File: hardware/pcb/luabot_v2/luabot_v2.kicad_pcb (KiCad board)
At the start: 2 copper layers, 60.3 x 29.8 mm, 21 parts, among them CON1 BAT_IN, P2 GND_GPIO, P3 VCC_GPIO, SW1 RESET, U1 ESP-07V2, U2 LM1117

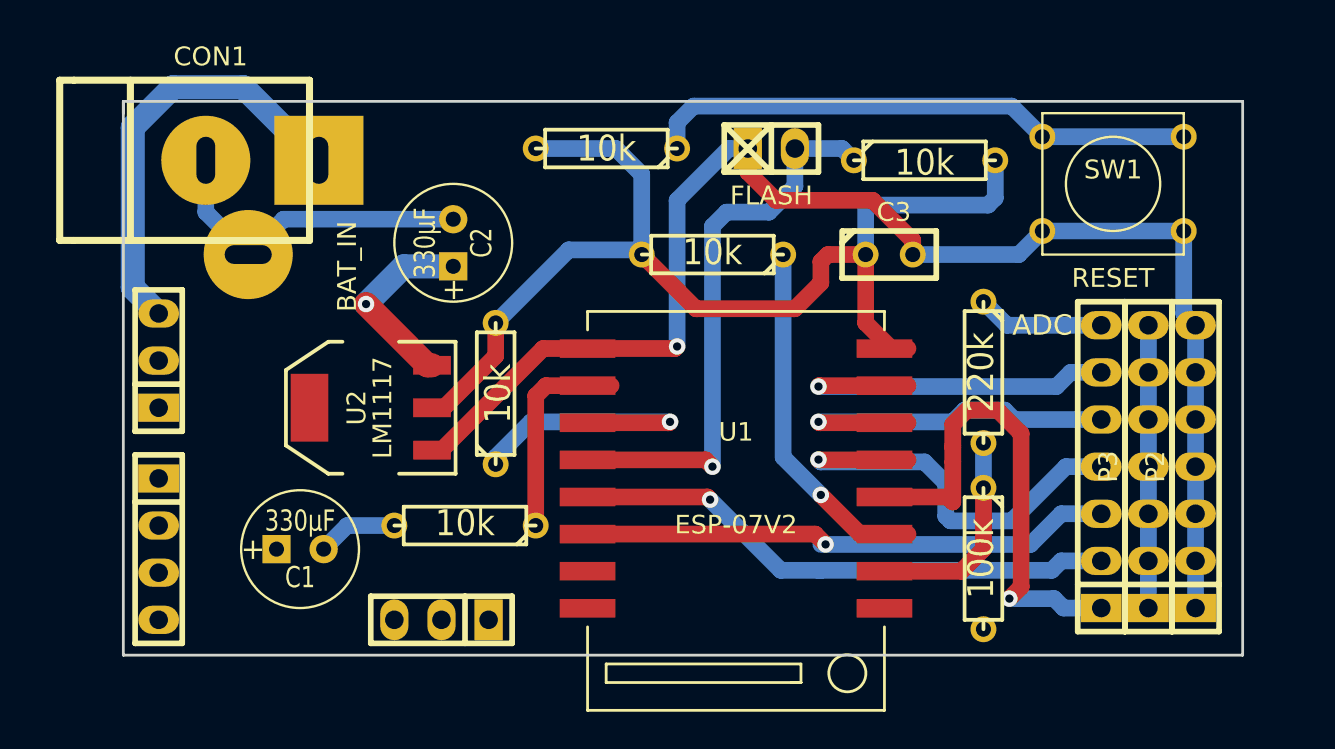
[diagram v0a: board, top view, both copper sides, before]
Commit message: avance hadware tarjeta terminada
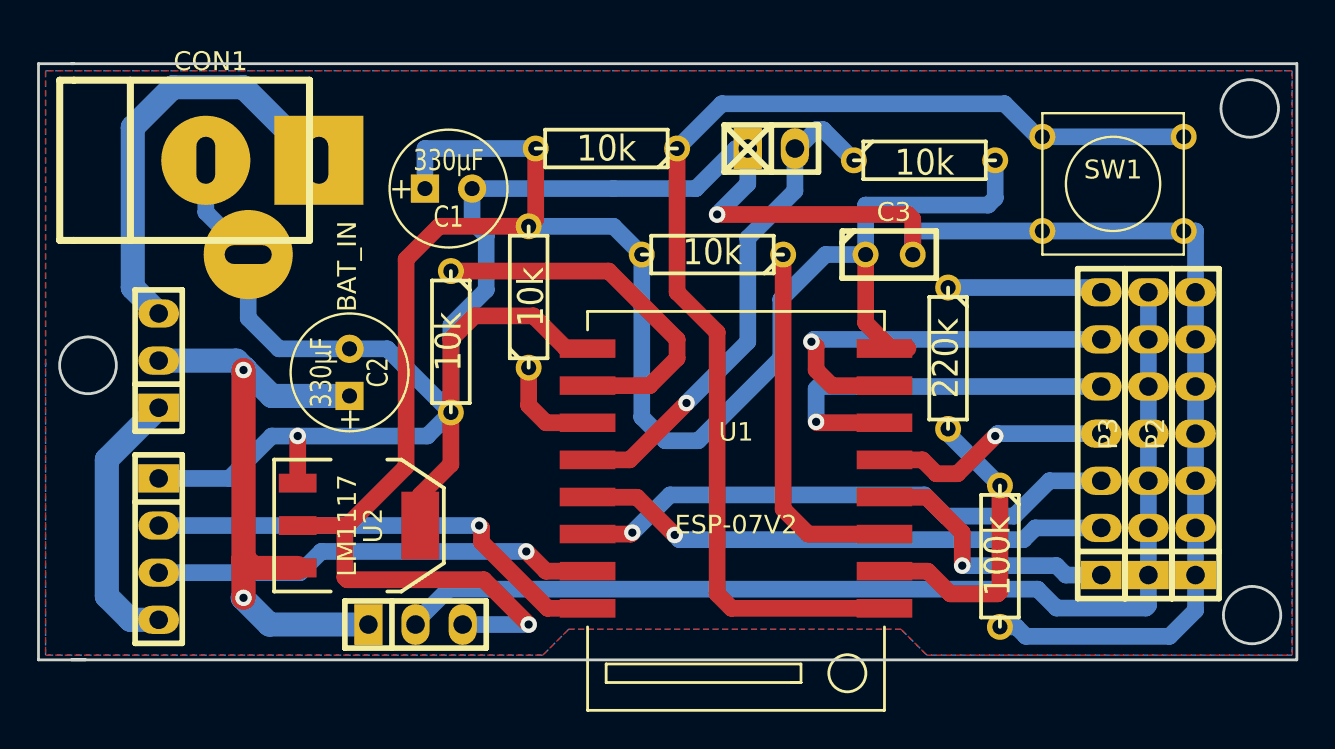
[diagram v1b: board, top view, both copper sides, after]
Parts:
- moved C1 21.0 mm to (41.0, 25.7)
- moved R3 9.94 mm to (41.1, 33.9), turned to 270 degrees
- moved C2 8.95 mm to (35.7, 35.6)
- moved U2 6.38 mm to (36.2, 43.8), turned to 270 degrees
- moved R5 5.50 mm to (45.3, 31.5)
- moved R7 2.05 mm to (67.9, 34.8)
- moved ADC 1.78 mm to (76.2, 38.9)
- moved P2 1.78 mm to (81.3, 38.9)
- moved P3 1.78 mm to (78.7, 38.9)
- moved 3.3V 1.42 mm to (39.2, 49.1), turned to 0 degrees
- moved R6 0.90 mm to (70.7, 45.5)
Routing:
- net GND: track 98.7 -> 155.5 mm, vias 1 -> 2
- net +3.3V: track 60.1 -> 107.9 mm
- net N-0000021: track 15.2 -> 57.7 mm
- net Reset: track 29.8 -> 63.3 mm
- net TX: track 0.00 -> 25.4 mm, vias 0 -> 1
- net +5V: track 10.5 -> 35.2 mm, vias 1 -> 2
- net RX: track 0.00 -> 24.0 mm, vias 0 -> 1
- net +5V_USB: track 0.00 -> 14.6 mm
- net D0: track 25.6 -> 14.5 mm
- net D5: track 23.7 -> 12.9 mm
- net O02: track 15.0 -> 5.60 mm, vias 1 -> 0
- net O15: track 11.3 -> 20.2 mm
- net ADC: track 10.3 -> 16.7 mm
- net FLASH: track 30.6 -> 27.0 mm
- net D2: track 27.6 -> 29.8 mm
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- added copper zone on B.Cu, net GND
- added copper zone on F.Cu, net GND
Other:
- board size 60.3 x 29.8 mm -> 67.8 x 32.1 mm
- board text added: "ADC"
- board text added: "FLASH"
- board text added: "RESET"
- board text added: "VCC"
